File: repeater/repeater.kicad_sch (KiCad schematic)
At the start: 8 parts, among them J1 blanking, J2 dev1, J3 Barrel_Jack, Q1 PN2222A, Q2 PN2222A

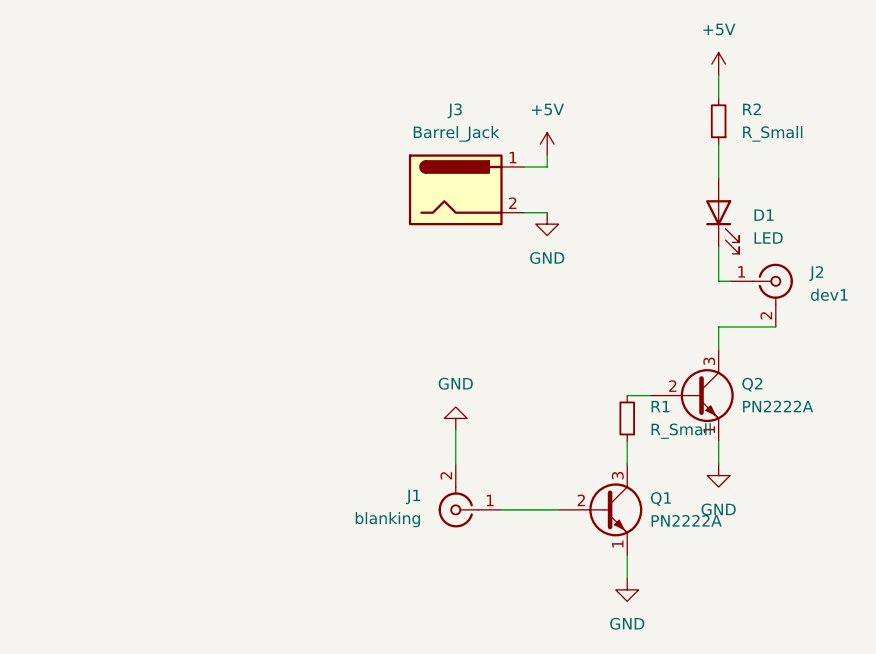
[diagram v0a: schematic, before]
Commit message: correct mistake
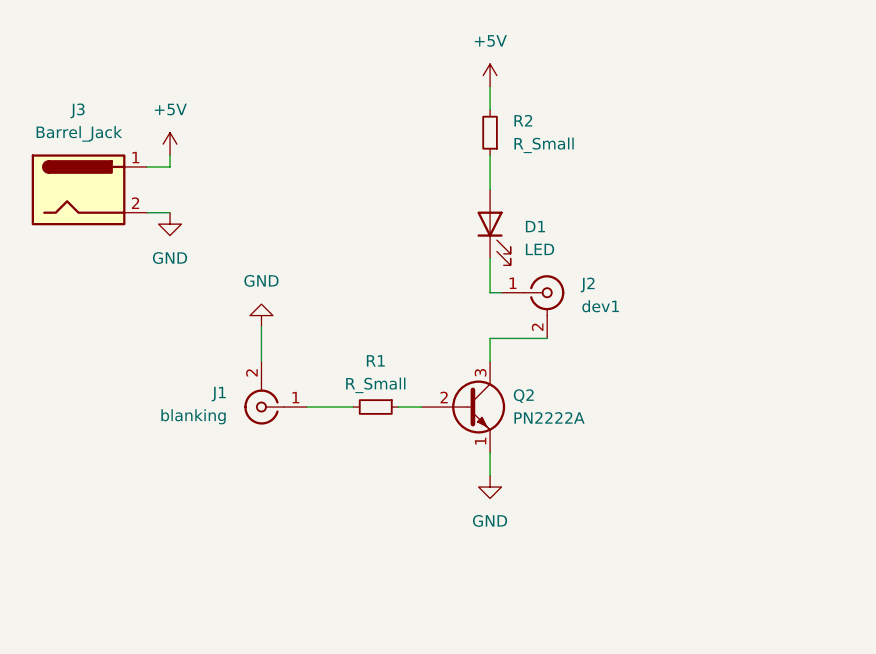
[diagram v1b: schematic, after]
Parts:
- removed Q1: PN2222A, Package_TO_SOT_THT:TO-92_Inline, symbol Transistor_BJT:PN2222A
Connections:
- net at Q2.2 (B): now also R1.1; no longer R1.2
- net at J1.1 (In): now also R1.2
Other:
- moved on the sheet: D1, J1, J2, J3, Q2, R1, R2
